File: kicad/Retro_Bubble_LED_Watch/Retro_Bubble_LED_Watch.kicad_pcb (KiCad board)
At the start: 2 copper layers, 35 x 35 mm, 24 parts, among them J1 ISP Programming Connector, J2 Pad Connector, SW1 KMS231G, SW2 KMS231G, U1 ATmega328PB-A, U2 DS1337S+

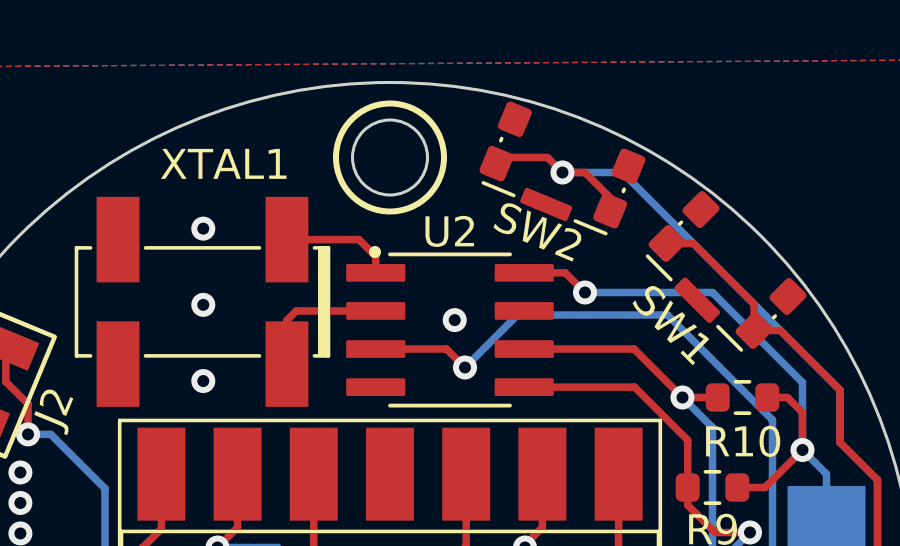
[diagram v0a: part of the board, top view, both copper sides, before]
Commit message: improved schematic readability + fixed component paths
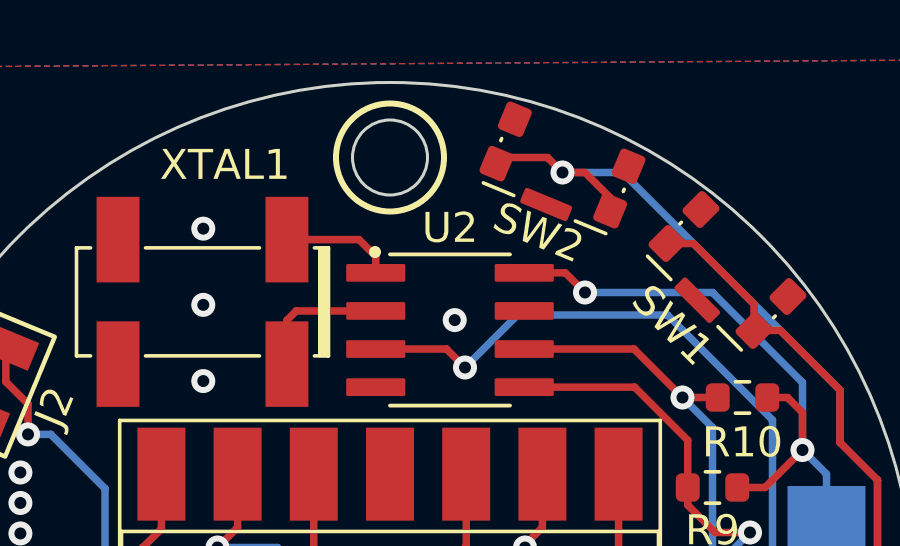
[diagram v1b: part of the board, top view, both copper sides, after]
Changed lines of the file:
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@@
     (property "Sheetname" "")
     (attr smd)
-    (fp_text reference "U2" (at 0 -3.25) (layer "F.SilkS")
-        (effects (font (size 1 1) (thickness 0.15)))
-    )
-    (fp_text value "DS1337S+" (at 6.71 2.832) (layer "F.Fab")
+    (fp_text reference "U2" (at 0 -3.4) (layer "F.SilkS")
+        (effects (font (size 1 1) (thickness 0.15)))
+    )
+    (fp_text value "DS1337S+" (at 7.46 3.332) (layer "F.Fab")
         (effects (font (size 1 1) (thickness 0.15)))
     )
@@
     (pad "8" smd roundrect (at 2.475 -1.905) (size 1.97 0.59) (layers "F.Cu" "F.Paste" "F.Mask") (roundrect_rratio 0.07)
       (net 16 "+BATT") (pinfunction "VCC") (pintype "power_in"))
-    (model "C:/Users/Szymon/Documents/KiCad/7.0/3dmodels/DS1337S_.step"
+    (model "${KIPRJMOD}/lib/models/DS1337S_.step"
       (offset (xyz 0 0 0))
       (scale (xyz 1 1 1))
@@
     (pad "14" smd rect (at 4.445 -7.62 90) (size 3.1 1.6) (layers "F.Cu" "F.Paste" "F.Mask")
       (net 14 "Net-(DS1-a)") (pinfunction "a") (pintype "input"))
-    (model "C:/Users/Szymon/Documents/Projects_Repository/Retro_Bubble_LED_Watch/models/step/HP5082-7415_with_SMD_Socket_assembly.stp"
-      (offset (xyz -3.75 7.75 1.5))
+    (model "${KIPRJMOD}/lib/models/HP5082-7415_with_SMD_Socket_assembly.stp"
+      (offset (xyz -3.8 7.5 1.5))
       (scale (xyz 1 1 1))
       (rotate (xyz 0 0 0))
@@
       (net 15 "GND") (pinfunction "2") (pintype "passive"))
     (pad "SH" smd roundrect (at 0 -1.425 157.5) (size 1.7 0.55) (layers "F.Cu" "F.Paste" "F.Mask") (roundrect_rratio 0.15))
-    (model "C:/Users/Szymon/Documents/KiCad/7.0/3dmodels/KMS231G.stp"
+    (model "${KIPRJMOD}/lib/models/KMS231G.stp"
       (offset (xyz 0 0 0))
       (scale (xyz 1 1 1))
@@
       (net 15 "GND") (pinfunction "2") (pintype "passive"))
     (pad "SH" smd roundrect (at 0 -1.425 135) (size 1.7 0.55) (layers "F.Cu" "F.Paste" "F.Mask") (roundrect_rratio 0.15))
-    (model "C:/Users/Szymon/Documents/KiCad/7.0/3dmodels/KMS231G.stp"
-      (offset (xyz 0 0 0))
-      (scale (xyz 1 1 1))
+    (model "${KIPRJMOD}/lib/models/KMS231G.stp"
+      (offset (xyz 0 0 0))
+      (scale (xyz 1 1 1))
